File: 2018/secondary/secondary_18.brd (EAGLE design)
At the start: 162.5 x 169.8 mm, 35 parts, among them Q1 BUZ11BV, Q2 BUZ11BV

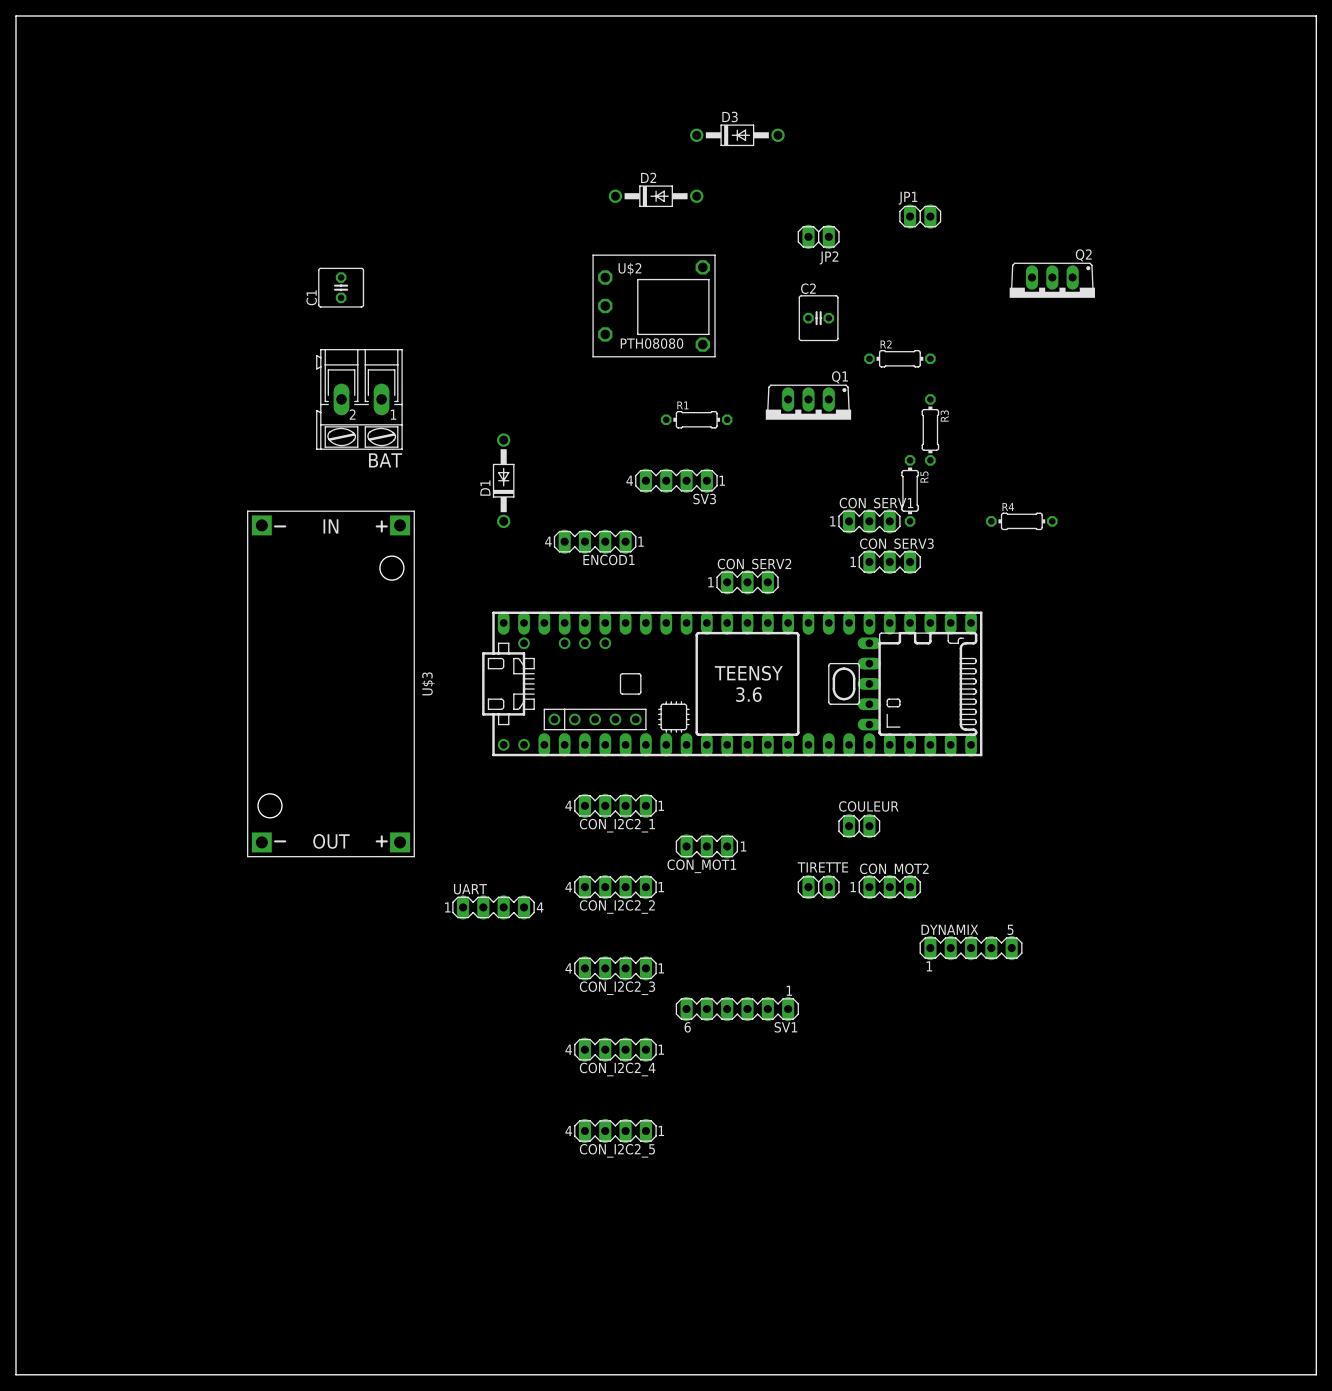
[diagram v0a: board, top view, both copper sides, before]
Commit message: [secondary] Adds the final board
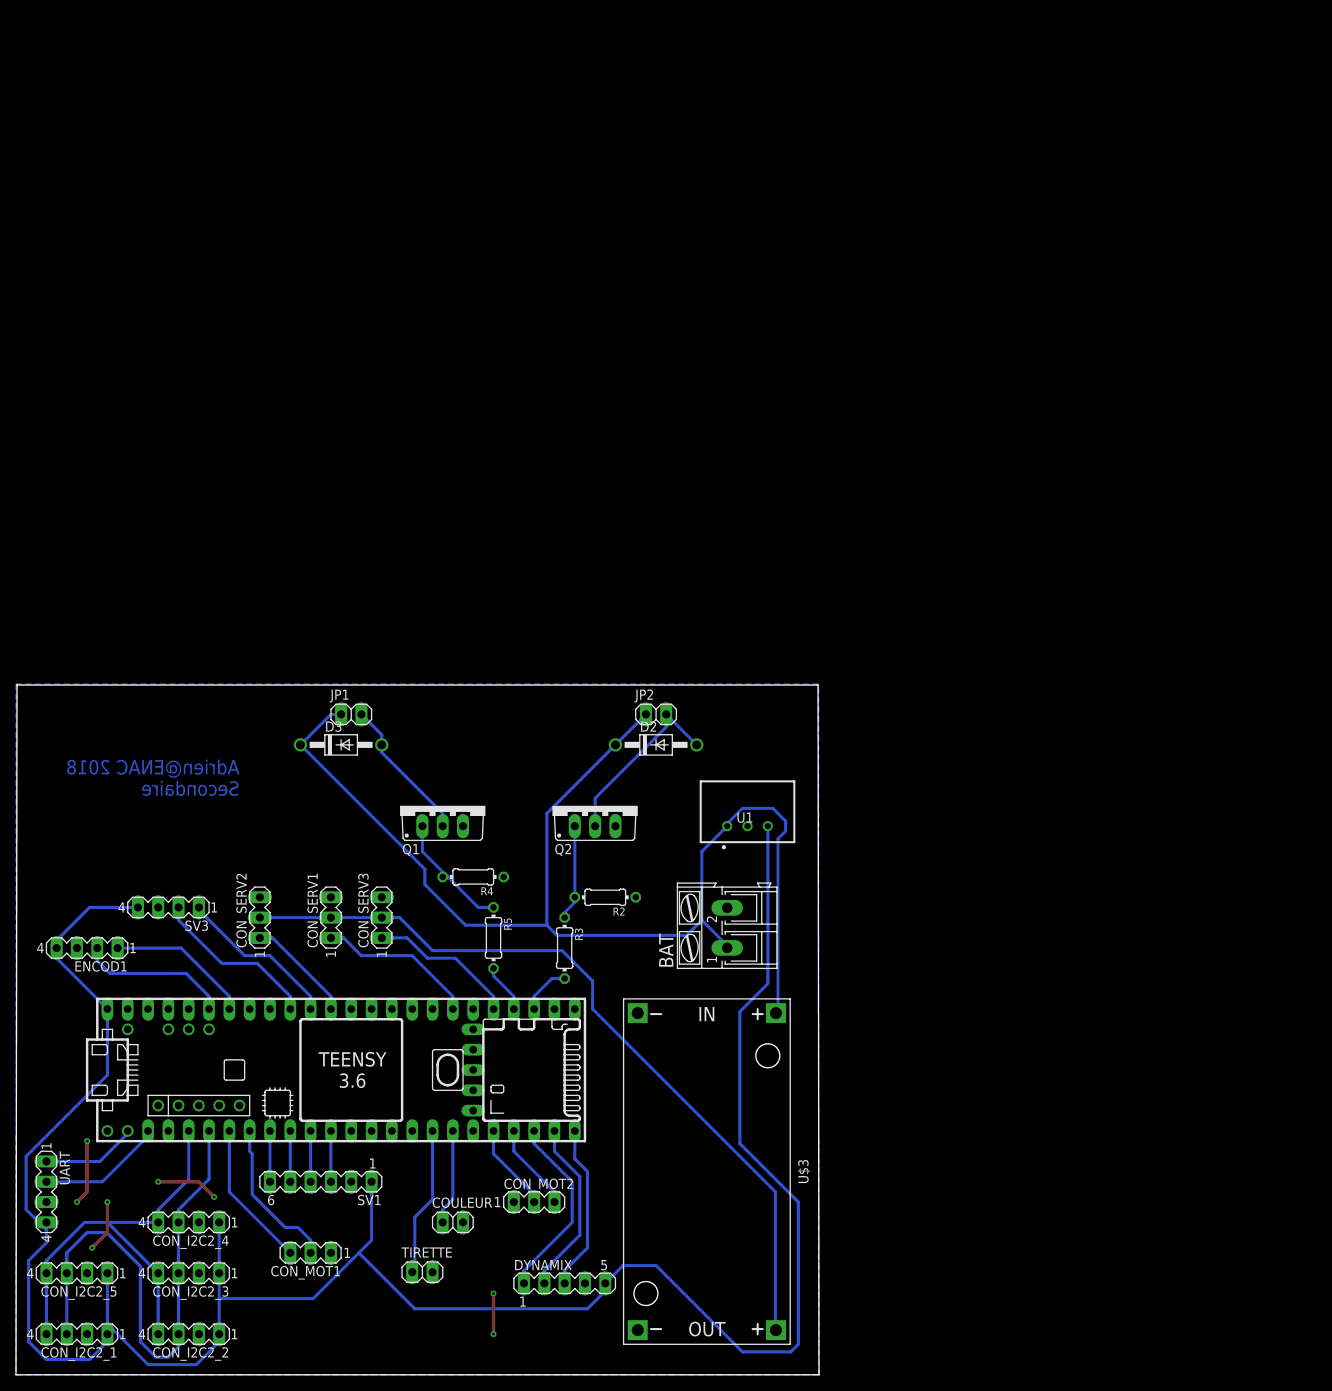
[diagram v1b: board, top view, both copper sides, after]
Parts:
- removed C1, C2: (no value), rcl:C025-060X050
- removed D1: 1N4004, diode:DO41-10
- removed R1: 348, resistor:0204/7
- removed U$2: PTH08080, pth08080:PTH08080EUF
- added U1: TSR_1-2450, SamacSys_Parts:TSR-1-24120
- moved JP1 94.5 mm to (41.9, 82.5)
- moved CON_I2C2_1 94.3 mm to (7.62, 5.08)
- moved D3 90.9 mm to (40.6, 78.7)
- moved Q2 85.4 mm to (72.4, 71.1), turned to 0 degrees
- moved CON_SERV1 83.6 mm to (39.4, 57.1), turned to 90 degrees
- moved SV3 82.9 mm to (19.1, 58.4)
- moved R4 81.7 mm to (57.1, 62.2), turned to 180 degrees
- moved ENCOD1 81.3 mm to (8.89, 53.3)
- moved BAT 80.3 mm to (88.9, 55.9), turned to 90 degrees
- moved R3 79.3 mm to (68.6, 53.3)
- moved CON_SERV3 77.5 mm to (45.7, 57.1), turned to 90 degrees
- moved CON_I2C2_2 77.3 mm to (21.6, 5.08)
- moved U$3 77.0 mm to (86.4, 25.4)
- moved R2 76.7 mm to (73.7, 59.7), turned to 180 degrees
- moved R5 76.4 mm to (59.7, 54.6)
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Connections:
- removed net N$1: R1.2, U$2.4
- net 12V: now also U1.1; no longer C2.2, D1.C, U$2.1
- net 5V_SIG: now also U1.3; no longer C1.1, D1.A, U$2.3
- net GND: now also U1.2; no longer C1.2, C2.1, R1.1, U$2.2
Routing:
- net 5V_SIG: track 0.00 -> 288.3 mm
- net 12V: track 0.00 -> 151.5 mm
- net 5V_PUI: track 0.00 -> 98.0 mm
- net N$23: track 0.00 -> 67.2 mm
- net N$21: track 0.00 -> 54.8 mm
- net GND: track 0.00 -> 27.5 mm, vias 0 -> 8
- net N$24: track 0.00 -> 23.5 mm
- net N$8: track 0.00 -> 23.0 mm
- net N$20: track 0.00 -> 22.2 mm
- net N$13: track 0.00 -> 21.1 mm
- net N$18: track 0.00 -> 20.9 mm
- net N$9: track 0.00 -> 20.3 mm
- net N$19: track 0.00 -> 19.9 mm
- net N$4: track 0.00 -> 19.3 mm
- net N$15: track 0.00 -> 19.0 mm
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- added copper zone on layer 16, net GND
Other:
- board size 162.5 x 169.8 mm -> 100.4 x 86.2 mm
- board text added: "Adrien@ENAC 2018 Secondaire"
